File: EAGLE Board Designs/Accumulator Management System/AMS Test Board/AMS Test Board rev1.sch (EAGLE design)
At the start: 41 parts, among them J1 CONNECTOR-2__B2B-PH-K, J10 CONNECTOR-2__B2B-PH-K, J11 CONNECTOR-2__B2B-PH-K, J12 CONNECTOR-2__B2B-PH-K, J13 CONNECTOR-2__B2B-PH-K, J14 CONNECTOR-2__B2B-PH-K, J15 CONNECTOR-2__B2B-PH-K, J16 CONNECTOR-2__B2B-PH-K, J17 CONNECTOR-2__B2B-PH-K, J18 CONNECTOR-2__B2B-PH-K, J19 CONNECTOR-2__B2B-PH-K, J2 CONNECTOR-2__B2B-PH-K, J20 CONNECTOR-2__B2B-PH-K, J22 CONNECTOR-1_5222, J23 CONNECTOR-1_5222, J24 CONNECTOR-1_5222, J25 CONNECTOR-1_5222, J26 CONNECTOR-1_5222, J27 CONNECTOR-1_5222, J28 CONNECTOR-1_5222, J29 CONNECTOR-1_5222, J3 CONNECTOR-2__B2B-PH-K, J30 CONNECTOR-1_5222, J31 CONNECTOR-1_5222, J32 CONNECTOR-1_5222, J33 CONNECTOR-1_5222, J34 CONNECTOR-1_5222, J35 CONNECTOR-1_5222, J36 CONNECTOR-1_5222, J37 CONNECTOR-1_5222, J38 CONNECTOR-1_5222, J39 CONNECTOR-1_5222, J4 CONNECTOR-2__B2B-PH-K, J40 CONNECTOR-1_5222, J41 CONNECTOR-1_5222, J42 CONNECTOR-1_5222, J5 CONNECTOR-2__B2B-PH-K, J6 CONNECTOR-2__B2B-PH-K, J7 CONNECTOR-2__B2B-PH-K, J8 CONNECTOR-2__B2B-PH-K, J9 CONNECTOR-2__B2B-PH-K

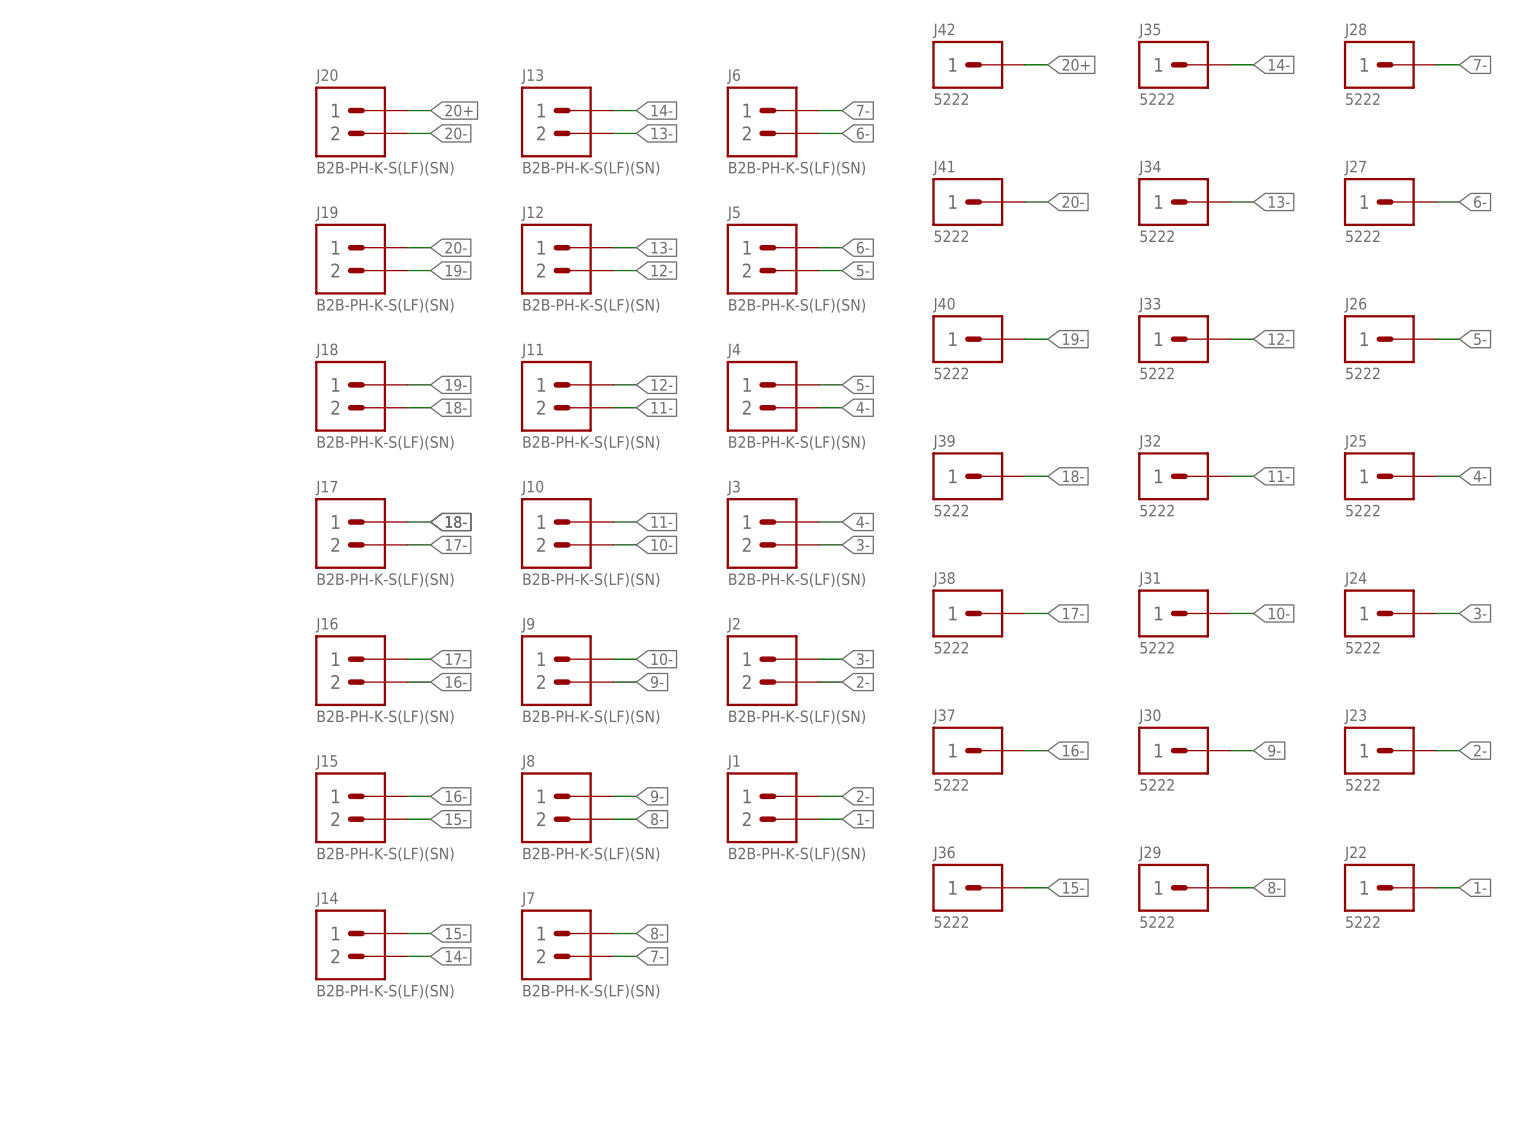
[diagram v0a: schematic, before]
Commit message: Update
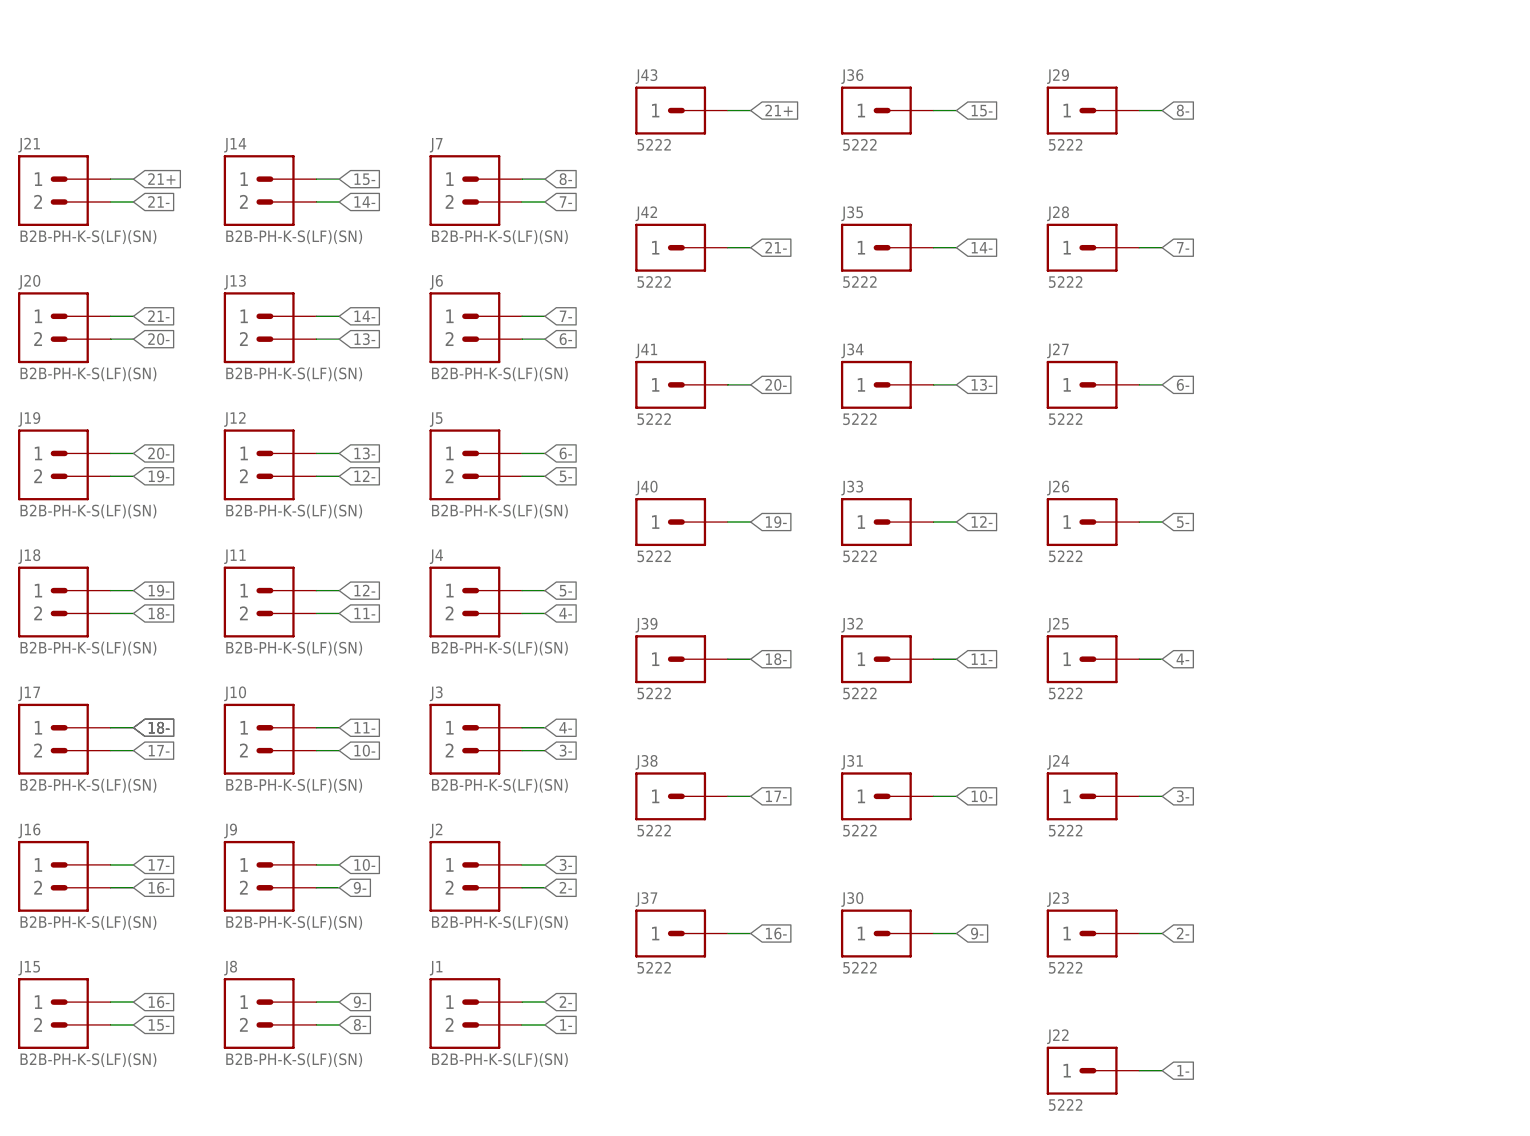
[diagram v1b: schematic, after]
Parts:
- added J21: CONNECTOR-2__B2B-PH-K, HyTechDevices:CONNECTOR-2__B2B-PH-K
- added J43: CONNECTOR-1_5222, HyTechDevices:CONNECTOR-1_5222
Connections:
- removed net 20+: J20.1, J42.1
- new net 21+: J21.1, J43.1
- new net 21-: J20.1, J21.2, J42.1
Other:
- moved on the sheet: J1, J10, J11, J12, J13, J14, J15, J16, J17, J18, J19, J2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
